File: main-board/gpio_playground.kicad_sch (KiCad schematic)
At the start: 31 parts, among them J1 Conn_02x04_Odd_Even, SW4 SW_Push, SW6 SW_Push, SW7 SW_Push, U16 BIWIN_DTS04GE_SMD, U17 74AHC244, U18 74AHCT1G08, U19 74AHCT1G08, U20 74AHC1G04

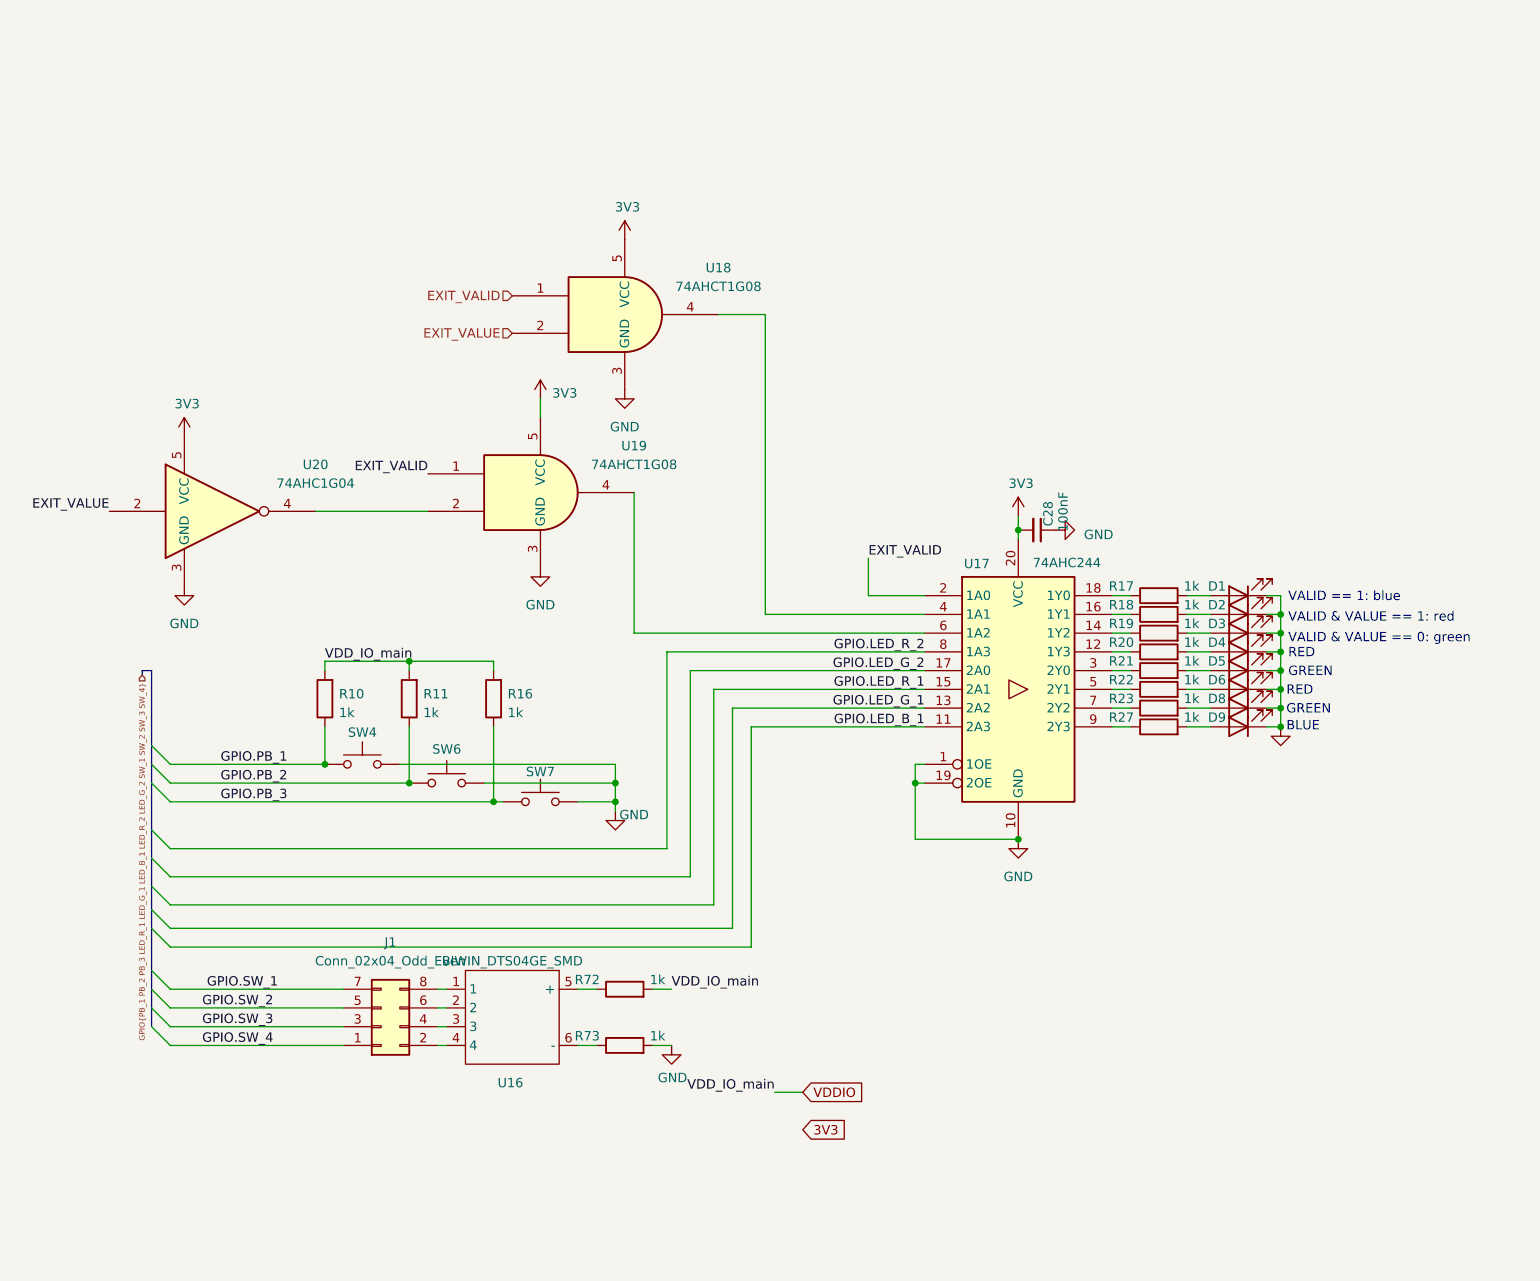
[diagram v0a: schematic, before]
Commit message: Testing board final version & production data
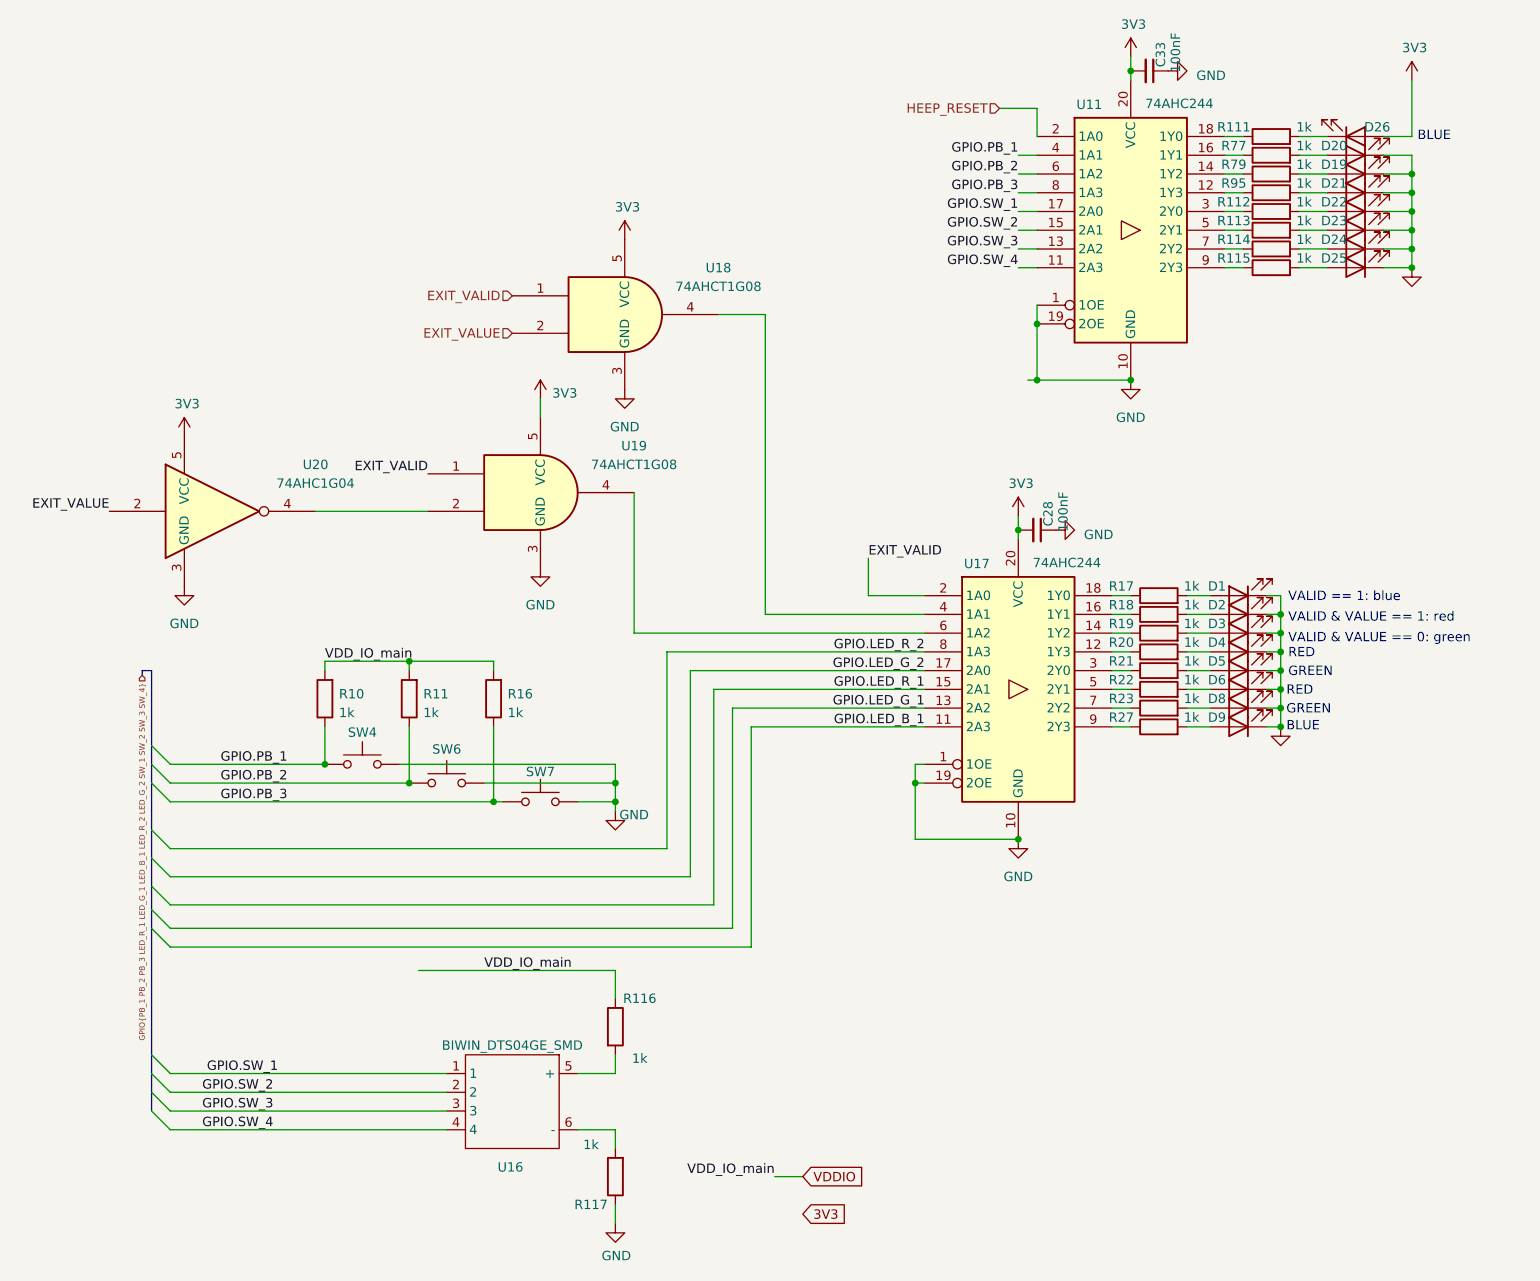
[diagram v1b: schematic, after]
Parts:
- removed J1: Conn_02x04_Odd_Even, Connector_PinHeader_2.54mm:PinHeader_2x04_P2.54mm_Vertical_SMD, symbol Connector_Generic:Conn_02x04_Odd_Even
- removed R72, R73: 1k, Resistor_SMD:R_0603_1608Metric, symbol Device:R
- added C33: 100nF, Capacitor_SMD:C_0603_1608Metric, symbol Device:C_Small
- added D19, D20, D21, D22, D23, D24, D25, D26: LED, LED_SMD:LED_0603_1608Metric, symbol Device:LED
- added R111, R112, R113, R114, R115, R116, R117, R77, R79, R95: 1k, Resistor_SMD:R_0603_1608Metric, symbol Device:R
- added U11: 74AHC244, Package_SO:TSSOP-20_4.4x6.5mm_P0.65mm, symbol 74xx:74AHC244
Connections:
- net 3V3: now also C33.2, D26.2 (A), U11.20 (VCC)
- net GND: now also C33.1, D19.1 (K), D20.1 (K), D21.1 (K), D22.1 (K), D23.1 (K), D24.1 (K), D25.1 (K), R117.1, U11.1 (1OE), U11.10 (GND), U11.19 (2OE)
- net GPIO.PB_1: now also U11.4 (1A1)
- net GPIO.PB_2: now also U11.6 (1A2)
- net GPIO.PB_3: now also U11.8 (1A3)
- net GPIO.SW_1: now also U16.1, U11.17 (2A0)
- net GPIO.SW_2: now also U16.2, U11.15 (2A1)
- net GPIO.SW_3: now also U16.3, U11.13 (2A2)
- net GPIO.SW_4: now also U16.4, U11.11 (2A3)
- net VDDIO: now also R116.1
- net at U16.6 (-): now also R117.2
- net at U16.5 (+): now also R116.2
- new net: R79.1, U11.14 (1Y2)
- new net: D19.2 (A), R79.2
- new net: D22.2 (A), R112.2
- new net: R95.1, U11.12 (1Y3)
- new net: R77.1, U11.16 (1Y1)
- new net: R111.1, U11.18 (1Y0)
- new net: R112.1, U11.3 (2Y0)
- new net: R113.1, U11.5 (2Y1)
- new net: R114.1, U11.7 (2Y2)
- new net: R115.1, U11.9 (2Y3)
- new net: D21.2 (A), R95.2
- new net: D20.2 (A), R77.2
- new net: D23.2 (A), R113.2
- new net: D24.2 (A), R114.2
- new net: D25.2 (A), R115.2
- new net: D26.1 (K), R111.2
- new net HEEP_RESET: U11.2 (1A0)
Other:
- moved on the sheet: U16

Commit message: production files
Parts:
- D1, D9: LCSC C84266 -> C84263
- D3, D5, D8: LCSC C965804 -> C84263
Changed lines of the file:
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@@
 			)
 		)
-		(property "LCSC" "C84266"
+		(property "LCSC" "C84263"
 			(at 217.805 123.19 0)
 			(effects
@@
 			)
 		)
-		(property "LCSC" "C965804"
+		(property "LCSC" "C84263"
 			(at 217.805 120.65 0)
 			(effects
@@
 			)
 		)
-		(property "LCSC" "C965804"
+		(property "LCSC" "C84263"
 			(at 217.805 110.49 0)
 			(effects
@@
 			)
 		)
-		(property "LCSC" "C84266"
+		(property "LCSC" "C84263"
 			(at 217.805 105.41 0)
 			(effects
@@
 			)
 		)
-		(property "LCSC" "C965804"
+		(property "LCSC" "C84263"
 			(at 217.805 115.57 0)
 			(effects
